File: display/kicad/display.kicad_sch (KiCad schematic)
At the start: 117 parts, among them J1 Conn_01x07_Pin, J2 Conn_01x02_Pin, J3 Conn_01x02_Pin, J4 Conn_01x02_Pin, J5 pcie_98, U1 ADS1261BIRHBT, U2 ESD5344D-TP, U3 TPS7A2050PDBVR, U4 TPS7A2025PDBVRr, U6 TPS65135, U7 ADP7182AUJZ-5.0, U8 ADP7182AUJZ-2.5, U9 XC6206P332MR

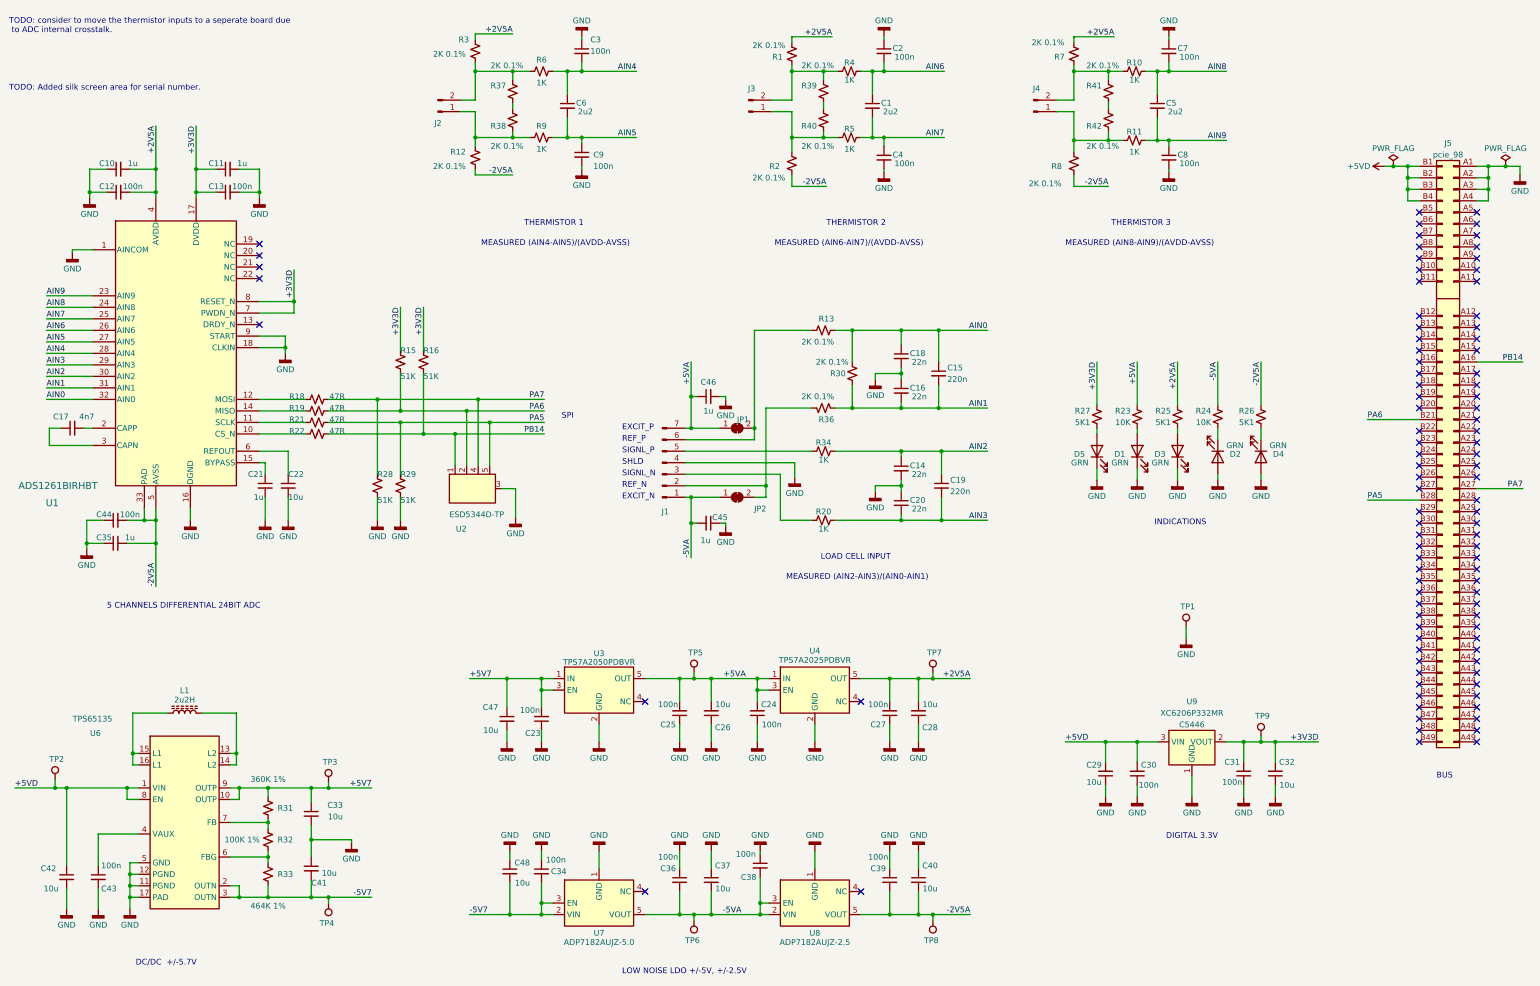
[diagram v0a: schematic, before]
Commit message: Work in progress on the display card.
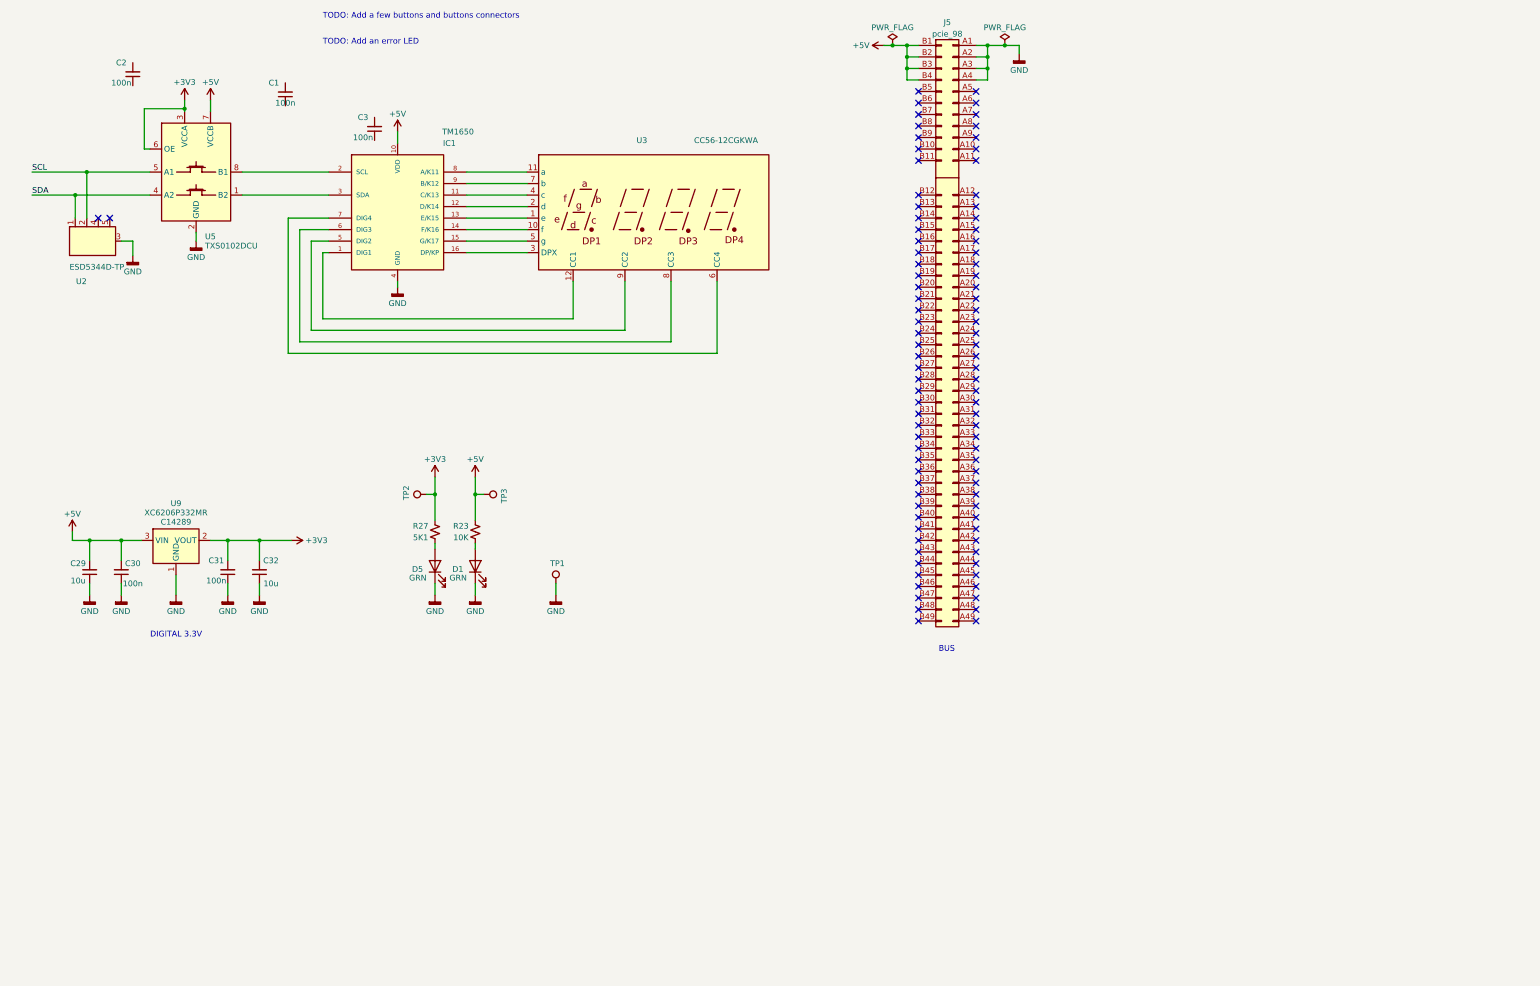
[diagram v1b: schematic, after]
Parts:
- removed C10, C11, C21, C35, C45, C46: 1u, Capacitor_SMD:C_0402_1005Metric, symbol Device:C_Small
- removed C12, C13, C23, C24, C25, C27, C34, C36, C38, C39, C4, C43, C44, C7, C8, C9: 100n, Capacitor_SMD:C_0402_1005Metric, symbol Device:C_Small
- removed C14, C16, C18, C20: 22n, Capacitor_SMD:C_0402_1005Metric, symbol Device:C_Small
- removed C15, C19: 220n, Capacitor_SMD:C_0402_1005Metric, symbol Device:C_Small
- removed C17: 4n7, Capacitor_SMD:C_0402_1005Metric, symbol Device:C_Small
- removed C22, C26, C28, C33, C37, C40, C41, C42, C47, C48: 10u, Capacitor_SMD:C_0603_1608Metric, symbol Device:C_Small
- removed C5, C6: 2u2, Capacitor_SMD:C_0402_1005Metric, symbol Device:C_Small
- removed D2, D3, D4: GRN, LED_SMD:LED_0603_1608Metric, symbol Device:LED
- removed J1: Conn_01x07_Pin, display:connector_7pins_horizontal, symbol Connector:Conn_01x07_Pin
- removed J2, J3, J4: Conn_01x02_Pin, display:connector_2pins_horizontal, symbol Connector:Conn_01x02_Pin
- removed JP1, JP2: SolderJumper_2_Bridged, Jumper:SolderJumper-2_P1.3mm_Bridged_Pad1.0x1.5mm, symbol Jumper:SolderJumper_2_Bridged
- removed L1: 2u2H, display:Inductor_C329578, symbol Device:L_Ferrite
- removed R1, R12, R13, R2, R3, R30, R36, R37, R38, R39, R40, R41, R42, R7, R8: 2K 0.1%, Resistor_SMD:R_0402_1005Metric, symbol Device:R_Small_US
- removed R10, R11, R20, R34, R4, R5, R6, R9: 1K, Resistor_SMD:R_0402_1005Metric, symbol Device:R_Small_US
- removed R15, R16, R28, R29: 51K, Resistor_SMD:R_0402_1005Metric, symbol Device:R_Small_US
- removed R18, R19, R21, R22: 47R, Resistor_SMD:R_0402_1005Metric, symbol Device:R_Small_US
- removed R24: 10K, Resistor_SMD:R_0402_1005Metric, symbol Device:R_Small_US
- removed R25, R26: 5K1, Resistor_SMD:R_0402_1005Metric, symbol Device:R_Small_US
- removed R31: 360K 1%, Resistor_SMD:R_0402_1005Metric, symbol Device:R_Small_US
- removed R32: 100K 1%, Resistor_SMD:R_0402_1005Metric, symbol Device:R_Small_US
- removed R33: 464K 1%, Resistor_SMD:R_0402_1005Metric, symbol Device:R_Small_US
- removed TP4, TP5, TP6, TP7, TP8, TP9: TestPoint, common:Test_Pad, symbol common:TestPoint
- removed U1: ADS1261BIRHBT, display:RHB0032E, symbol display:ADS1261IRHBR
- removed U3: TPS7A2050PDBVR, display:SOT-23-5, symbol display:TPS7A2050
- removed U4: TPS7A2025PDBVRr, display:SOT-23-5, symbol display:TPS7A2050
- removed U6: TPS65135, display:WQFN-16-1EP_3x3mm_P0.5mm_EP1.68x1.68mm_ThermalVias, symbol display:TPS65135
- removed U7: ADP7182AUJZ-5.0, Package_TO_SOT_SMD:TSOT-23-5, symbol display:ADP7182AUJZ
- removed U8: ADP7182AUJZ-2.5, Package_TO_SOT_SMD:TSOT-23-5, symbol display:ADP7182AUJZ
- added IC1: TM1650, Package_SO:SOP-16_3.9x9.9mm_P1.27mm, symbol display:TM1650
- added U3: CC56-12CGKWA, Display_7Segment:CA56-12CGKWA, symbol display:CC56-12CGKWA
- added U5: TXS0102DCU, Package_SO:VSSOP-8_2.3x2mm_P0.5mm, symbol display:TXS0102DCU
- C1: value 2u2 -> 100n; LCSC C12530 -> C1525
- U9: footprint Package_TO_SOT_SMD:SOT-23-3 -> Package_TO_SOT_SMD:SOT-89-3; symbol breakout:XC6206P332MR -> display:XC6206P332MR; LCSC C5446 -> C14289
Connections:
- net +5VA is gone; now on net +5V: R23.1
- net GND: now also IC1.4 (GND), U5.2 (GND); no longer C2.1, C3.1
- net +3V3D renamed +3V3
- net +3V3: now also TP2.1, U5.3 (VCCA), U5.6 (OE)
- net +5V7 renamed +5V
- net +5V: now also C29.2, C30.2, J5.B1 (Pin_b1), J5.B2 (Pin_b2), J5.B3 (Pin_b3), J5.B4 (Pin_b4), U9.3 (VIN), IC1.10 (VDD), U5.7 (VCCB)
- removed net +5VD: C29.2, C30.2, J5.B1 (Pin_b1), J5.B2 (Pin_b2), J5.B3 (Pin_b3), J5.B4 (Pin_b4), TP2.1, U9.3 (VIN)
- net AIN4: no longer names the net of C3.2
- net AIN6: no longer names the net of C1.1
- net AIN6: no longer C2.2
- net AIN7: no longer names the net of C1.2
- net PA5: no longer names the net of U2.5 (D4)
- net PA5: no longer J5.B28 (Pin_b28)
- net PA6: no longer names the net of J5.B21 (Pin_b21)
- net PA6: no longer U2.2 (D2)
- net PA7: no longer names the net of U2.4 (D3)
- net PA7: no longer J5.A27 (Pin_a27)
- net PB14: no longer names the net of J5.A16 (Pin_a16)
- net PB14: no longer U2.1 (D1)
- new net: IC1.13 (E/K15), U3.1 (e)
- new net: IC1.14 (F/K16), U3.10 (f)
- new net: IC1.8 (A/K11), U3.11 (a)
- new net: IC1.1 (DIG1), U3.12 (CC1)
- new net: IC1.12 (D/K14), U3.2 (d)
- new net: IC1.16 (DP/KP), U3.3 (DPX)
- new net: IC1.11 (C/K13), U3.4 (c)
- new net: IC1.15 (G/K17), U3.5 (g)
- new net: IC1.7 (DIG4), U3.6 (CC4)
- new net: IC1.9 (B/K12), U3.7 (b)
- new net: IC1.6 (DIG3), U3.8 (CC3)
- new net: IC1.5 (DIG2), U3.9 (CC2)
- new net: IC1.2 (SCL), U5.8 (B1)
- new net: IC1.3 (SDA), U5.1 (B2)
- new net SCL: U2.2 (D2), U5.5 (A1)
- new net SDA: U2.1 (D1), U5.4 (A2)
- no-connect marks 95 -> 92
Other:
- note added: "TODO: Add a few buttons and buttons connectors"
- note added: "TODO: Add an error LED"
- note removed: "5 CHANNELS DIFFERENTIAL 24BIT ADC"
- note removed: "DC/DC +/-5.7V"
- note removed: "EXCIT_N"
- note removed: "EXCIT_P"
- note removed: "INDICATIONS"
- note removed: "LOAD CELL INPUT"
- note removed: "LOW NOISE LDO +/-5V, +/-2.5V"
- note removed: "MEASURED (AIN2-AIN3)/(AIN0-AIN1)"
- note removed: "MEASURED (AIN4-AIN5)/(AVDD-AVSS)"
- note removed: "MEASURED (AIN6-AIN7)/(AVDD-AVSS)"
- note removed: "MEASURED (AIN8-AIN9)/(AVDD-AVSS)"
- note removed: "REF_N"
- note removed: "REF_P"
- note removed: "SHLD"
- note removed: "SIGNL_N"
- note removed: "SIGNL_P"
- note removed: "SPI"
- note removed: "THERMISTOR 1"
- note removed: "THERMISTOR 2"
- note removed: "THERMISTOR 3"
- note removed: "TODO: Added silk screen area for serial number."
- note removed: "TODO: consider to move the thermistor inputs to a seperate board due to ADC internal crosstalk."
- moved on the sheet: C29, C30, C31, C32, D1, D5, J5, R23, R27, TP1, U2, U9

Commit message: More progress on the Display board.
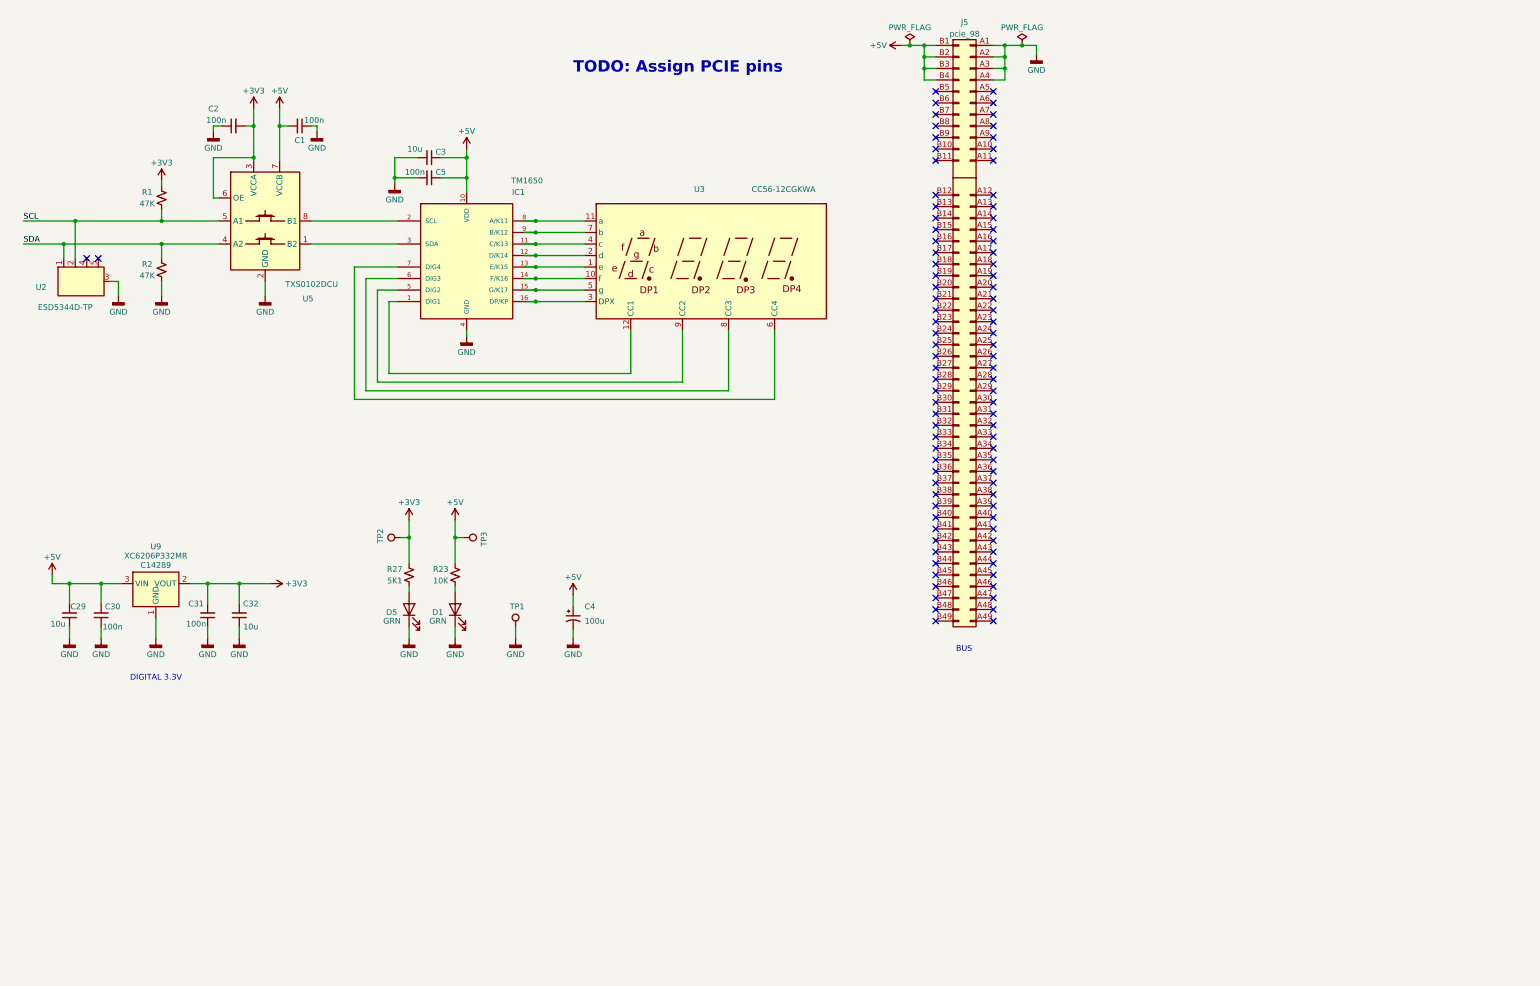
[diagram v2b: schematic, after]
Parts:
- added C4: 100u, symbol Device:C_Polarized_Small_US
- added C5: 100n, Capacitor_SMD:C_0402_1005Metric, symbol Device:C_Small
- added R1, R2: 47K, Resistor_SMD:R_0402_1005Metric, symbol Device:R_Small_US
- C3: value 100n -> 10u; LCSC C1525 -> (none)
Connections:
- net +3V3: now also C2.2, R1.1
- net +5V: now also C1.2, C3.1, C4.1, C5.1
- net GND: now also C1.1, C2.1, C3.2, C4.2, C5.2, R2.2
- net SCL: now also R1.2
- net SDA: now also R2.1
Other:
- note added: "TODO: Assign PCIE pins"
- note removed: "TODO: Add a few buttons and buttons connectors"
- note removed: "TODO: Add an error LED"
- title: ADS1261B ADC BOARD -> DISPLAY BOARD
- moved on the sheet: C1, C2, C29, C3, C30, C31, C32, D1, D5, IC1, J5, R23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
